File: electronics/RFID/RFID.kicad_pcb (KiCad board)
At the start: 2 copper layers, 48.3 x 71.1 mm, 22 parts, among them J1 USB_C_Receptacle_PowerOnly_6P, J2 Conn deur, J3 Conn Uart, J4 Conn_01x16_Pin, J5 Conn motion, U1 AP63202WU, U2 74LVC2G14

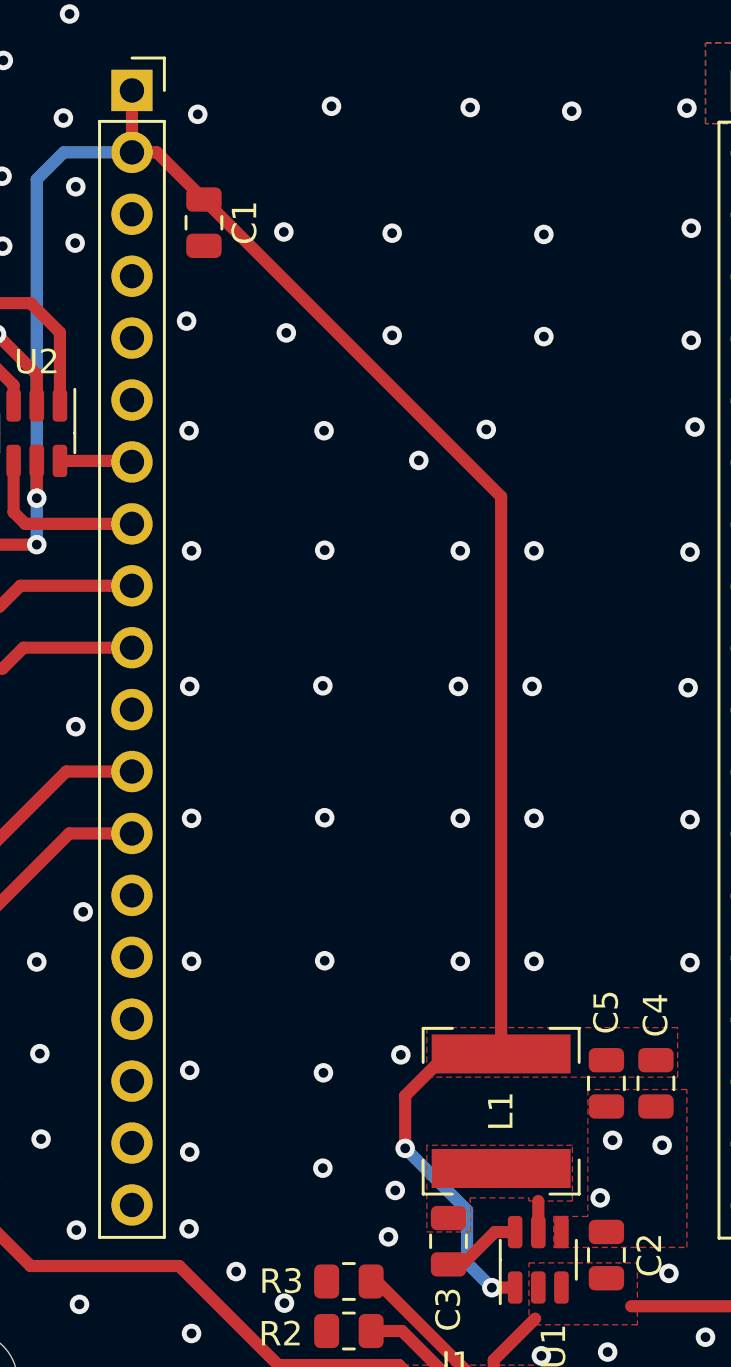
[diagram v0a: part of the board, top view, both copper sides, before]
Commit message: proxima fixed :chad:
fixed by proxi hihihiih love you <3
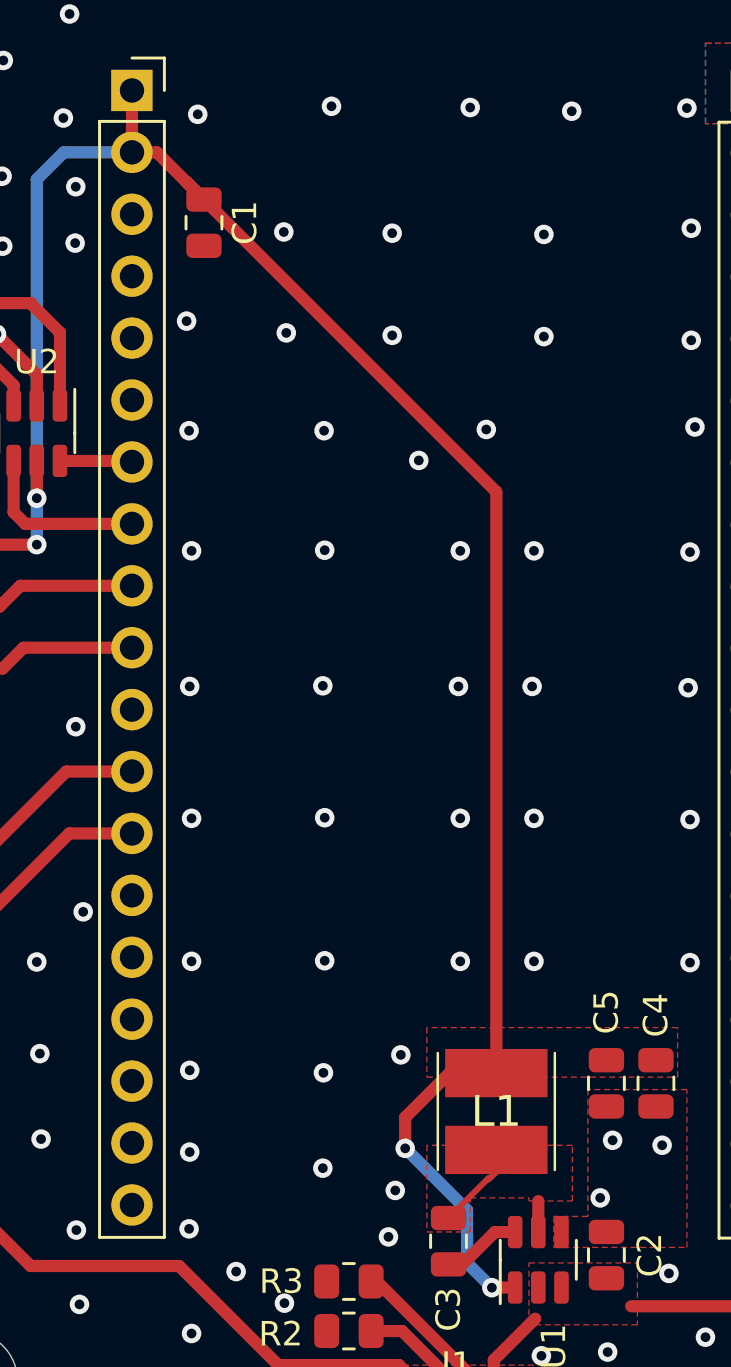
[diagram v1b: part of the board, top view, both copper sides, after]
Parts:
- L1: footprint Inductor_SMD:L_Bourns-SRN6028 -> KiCad:SRR4828A3R9Y
- moved L1 0.20 mm to (119.7, 96.3), turned to 180 degrees
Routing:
- net Net-(U1-SW): track 1.28 -> 5.21 mm
- net +3.3V: track 86.5 -> 88.5 mm
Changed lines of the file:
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@@
   (net 43 "unconnected-(U3-D3-Pad17)")
   (net 44 "unconnected-(U3-0-Pad33)")
-  (footprint "Inductor_SMD:L_Bourns-SRN6028" (layer "F.Cu")
-    (at 119.888 96.266 90)
-    (descr "Bourns SRN6028 series SMD inductor")
-    (tags "Bourns SRN6028 SMD inductor")
+  (footprint "KiCad:SRR4828A3R9Y" (layer "F.Cu")
+    (at 119.689398 96.277231 180)
+    (descr "SRR4828A-3R9Y-2")
+    (tags "Inductor")
     (property "Sheetfile" "RFID.kicad_sch")
     (property "Sheetname" "")
@@
     (property "ki_keywords" "inductor choke coil reactor magnetic")
     (attr smd)
-    (fp_text reference "L1" (at 0 0 90) (layer "F.SilkS")
-        (effects (font (size 1 1) (thickness 0.15)))
-    )
-    (fp_text value "3.9µH" (at 0 -4 90) (layer "F.Fab")
-        (effects (font (size 1 1) (thickness 0.15)))
-    )
-    (fp_text user "${REFERENCE}" (at 0 0 90) (layer "F.Fab")
-        (effects (font (size 1 1) (thickness 0.15)))
-    )
-    (fp_line (start -3.4 -3.2) (end -3.4 -2)
-      (stroke (width 0.12) (type solid)) (layer "F.SilkS"))
-    (fp_line (start -3.4 -3.2) (end -2 -3.2)
-      (stroke (width 0.12) (type solid)) (layer "F.SilkS"))
-    (fp_line (start -3.4 3.2) (end -3.4 2)
-      (stroke (width 0.12) (type solid)) (layer "F.SilkS"))
-    (fp_line (start -3.4 3.2) (end -2 3.2)
-      (stroke (width 0.12) (type solid)) (layer "F.SilkS"))
-    (fp_line (start 3.4 -3.2) (end 2 -3.2)
-      (stroke (width 0.12) (type solid)) (layer "F.SilkS"))
-    (fp_line (start 3.4 -3.2) (end 3.4 -2)
-      (stroke (width 0.12) (type solid)) (layer "F.SilkS"))
-    (fp_line (start 3.4 3.2) (end 2 3.2)
-      (stroke (width 0.12) (type solid)) (layer "F.SilkS"))
-    (fp_line (start 3.4 3.2) (end 3.4 2)
-      (stroke (width 0.12) (type solid)) (layer "F.SilkS"))
-    (fp_line (start -3.3 -3.1) (end -3.3 3.1)
-      (stroke (width 0.05) (type solid)) (layer "F.CrtYd"))
-    (fp_line (start -3.3 -3.1) (end 3.3 -3.1)
-      (stroke (width 0.05) (type solid)) (layer "F.CrtYd"))
-    (fp_line (start 3.3 -3.1) (end 3.3 3.1)
-      (stroke (width 0.05) (type solid)) (layer "F.CrtYd"))
-    (fp_line (start 3.3 3.1) (end -3.3 3.1)
-      (stroke (width 0.05) (type solid)) (layer "F.CrtYd"))
-    (fp_line (start -3.3 -3.1) (end -3.3 3.1)
-      (stroke (width 0.1) (type solid)) (layer "F.Fab"))
-    (fp_line (start -3.3 -3.1) (end 3.3 -3.1)
-      (stroke (width 0.1) (type solid)) (layer "F.Fab"))
-    (fp_line (start 3.3 -3.1) (end 3.3 3.1)
-      (stroke (width 0.1) (type solid)) (layer "F.Fab"))
-    (fp_line (start 3.3 3.1) (end -3.3 3.1)
-      (stroke (width 0.1) (type solid)) (layer "F.Fab"))
-    (pad "1" smd rect (at -2.35 0 90) (size 1.6 5.7) (layers "F.Cu" "F.Paste" "F.Mask")
+    (fp_text reference "L1" (at 0 0) (layer "F.SilkS")
+        (effects (font (size 1.27 1.27) (thickness 0.254)))
+    )
+    (fp_text value "3.9µH" (at 0 0) (layer "F.SilkS") hide
+        (effects (font (size 1.27 1.27) (thickness 0.254)))
+    )
+    (fp_text user "${REFERENCE}" (at 0 0) (layer "F.Fab")
+        (effects (font (size 1.27 1.27) (thickness 0.254)))
+    )
+    (fp_line (start -2.4 -2.4) (end -2.4 2.4)
+      (stroke (width 0.1) (type solid)) (layer "F.SilkS"))
+    (fp_line (start 2.4 -2.4) (end 2.4 2.4)
+      (stroke (width 0.1) (type solid)) (layer "F.SilkS"))
+    (fp_line (start -3.4 -3.565) (end 3.4 -3.565)
+      (stroke (width 0.1) (type solid)) (layer "F.CrtYd"))
+    (fp_line (start -3.4 3.565) (end -3.4 -3.565)
+      (stroke (width 0.1) (type solid)) (layer "F.CrtYd"))
+    (fp_line (start 3.4 -3.565) (end 3.4 3.565)
+      (stroke (width 0.1) (type solid)) (layer "F.CrtYd"))
+    (fp_line (start 3.4 3.565) (end -3.4 3.565)
+      (stroke (width 0.1) (type solid)) (layer "F.CrtYd"))
+    (fp_line (start -2.4 -2.4) (end 2.4 -2.4)
+      (stroke (width 0.2) (type solid)) (layer "F.Fab"))
+    (fp_line (start -2.4 2.4) (end -2.4 -2.4)
+      (stroke (width 0.2) (type solid)) (layer "F.Fab"))
+    (fp_line (start 2.4 -2.4) (end 2.4 2.4)
+      (stroke (width 0.2) (type solid)) (layer "F.Fab"))
+    (fp_line (start 2.4 2.4) (end -2.4 2.4)
+      (stroke (width 0.2) (type solid)) (layer "F.Fab"))
+    (pad "1" smd rect (at 0 -1.575 270) (size 1.98 4.2) (layers "F.Cu" "F.Paste" "F.Mask")
       (net 4 "Net-(U1-SW)") (pinfunction "1") (pintype "passive"))
-    (pad "2" smd rect (at 2.35 0 90) (size 1.6 5.7) (layers "F.Cu" "F.Paste" "F.Mask")
+    (pad "2" smd rect (at 0 1.575 270) (size 1.98 4.2) (layers "F.Cu" "F.Paste" "F.Mask")
       (net 1 "+3.3V") (pinfunction "2") (pintype "passive"))
-    (model "${KICAD6_3DMODEL_DIR}/Inductor_SMD.3dshapes/L_Bourns-SRN6028.wrl"
+    (model "SRR4828A-3R9Y.stp"
       (offset (xyz 0 0 0))
       (scale (xyz 1 1 1))
@@
   )
   (segment (start 104.7434 54.3924) (end 104.7434 56.9324) (width 0.5) (layer "F.Cu") (net 1))
+  (segment (start 119.689398 70.860398) (end 119.689398 94.702231) (width 0.5) (layer "F.Cu") (net 1))
   (segment (start 100.838 73.025) (end 96.52 73.025) (width 0.5) (layer "F.Cu") (net 1))
-  (segment (start 115.951 95.631) (end 117.666 93.916) (width 0.5) (layer "F.Cu") (net 1))
-  (segment (start 119.888 71.059) (end 119.888 93.916) (width 0.5) (layer "F.Cu") (net 1))
-  (segment (start 105.7614 56.9324) (end 107.696 58.867) (width 0.5) (layer "F.Cu") (net 1))
-  (segment (start 117.666 93.916) (end 119.888 93.916) (width 0.5) (layer "F.Cu") (net 1))
-  (segment (start 107.696 58.867) (end 119.888 71.059) (width 0.5) (layer "F.Cu") (net 1))
+  (segment (start 117.768769 94.702231) (end 115.951 96.52) (width 0.5) (layer "F.Cu") (net 1))
   (segment (start 120.462 103.4995) (end 119.5125 103.4995) (width 0.5) (layer "F.Cu") (net 1))
+  (segment (start 119.666648 94.430447) (end 118.556648 94.430447) (width 0.5) (layer "F.Cu") (net 1))
+  (segment (start 119.689398 94.702231) (end 119.587029 94.8046) (width 0.5) (layer "F.Cu") (net 1))
+  (segment (start 115.951 96.52) (end 115.951 97.79) (width 0.5) (layer "F.Cu") (net 1))
+  (segment (start 106.9645 58.1355) (end 119.689398 70.860398) (width 0.5) (layer "F.Cu") (net 1))
+  (segment (start 105.7614 56.9324) (end 106.9645 58.1355) (width 0.5) (layer "F.Cu") (net 1))
   (segment (start 119.5125 103.4995) (end 119.507 103.505) (width 0.5) (layer "F.Cu") (net 1))
-  (segment (start 115.951 97.79) (end 115.951 95.631) (width 0.5) (layer "F.Cu") (net 1))
+  (segment (start 119.689398 94.702231) (end 117.768769 94.702231) (width 0.5) (layer "F.Cu") (net 1))
+  (segment (start 106.9645 58.1355) (end 107.696 58.867) (width 0.5) (layer "F.Cu") (net 1))
   (segment (start 104.7434 56.9324) (end 105.7614 56.9324) (width 0.5) (layer "F.Cu") (net 1))
   (segment (start 100.838 69.5905) (end 100.838 71.12) (width 0.5) (layer "F.Cu") (net 1))
@@
   (segment (start 132.715 101.092) (end 132.715 94.996) (width 0.5) (layer "B.Cu") (net 3))
   (segment (start 133.6675 94.0435) (end 135.763 91.948) (width 0.5) (layer "B.Cu") (net 3))
+  (segment (start 119.666648 98.773352) (end 119.38 99.06) (width 0.25) (layer "F.Cu") (net 4))
   (segment (start 121.412 101.2245) (end 121.412 99.949) (width 0.5) (layer "F.Cu") (net 4))
+  (segment (start 119.666648 97.580447) (end 119.666648 98.773352) (width 0.25) (layer "F.Cu") (net 4))
+  (segment (start 119.38 98.999) (end 117.729 100.65) (width 0.25) (layer "F.Cu") (net 4))
   (segment (start 118.303 102.55) (end 119.6285 101.2245) (width 0.5) (layer "F.Cu") (net 5))
   (segment (start 119.6285 101.2245) (end 120.462 101.2245) (width 0.5) (layer "F.Cu") (net 5))
